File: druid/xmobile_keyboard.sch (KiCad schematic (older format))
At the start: 34 parts

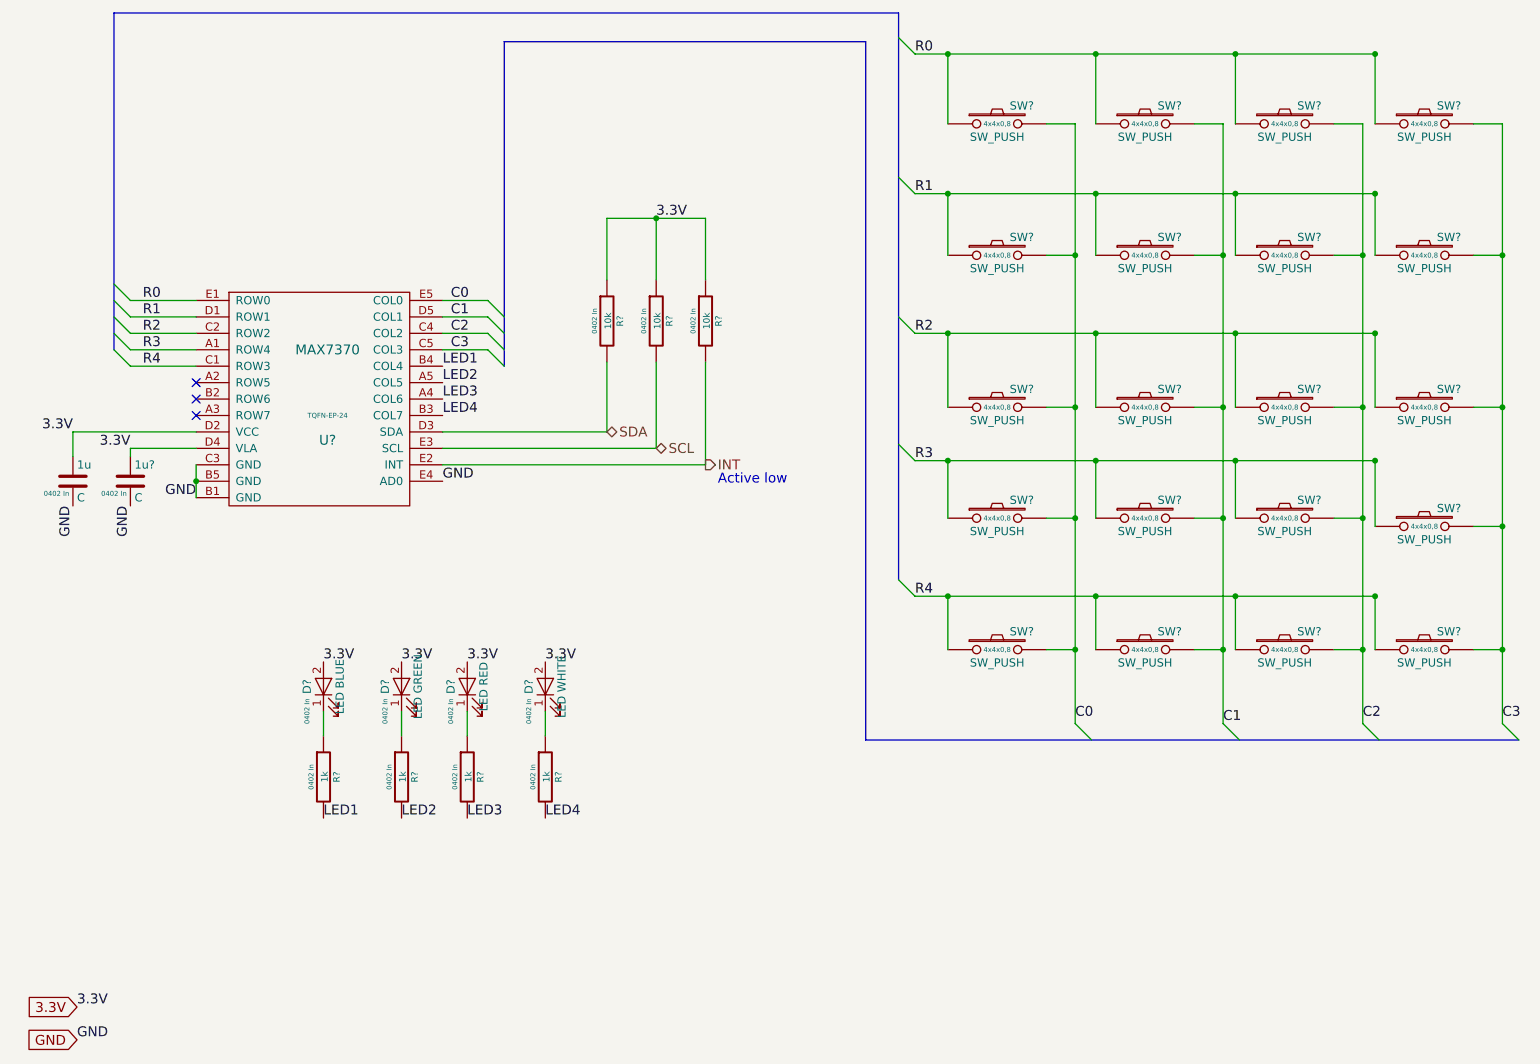
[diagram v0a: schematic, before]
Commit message: looks like all packages added.
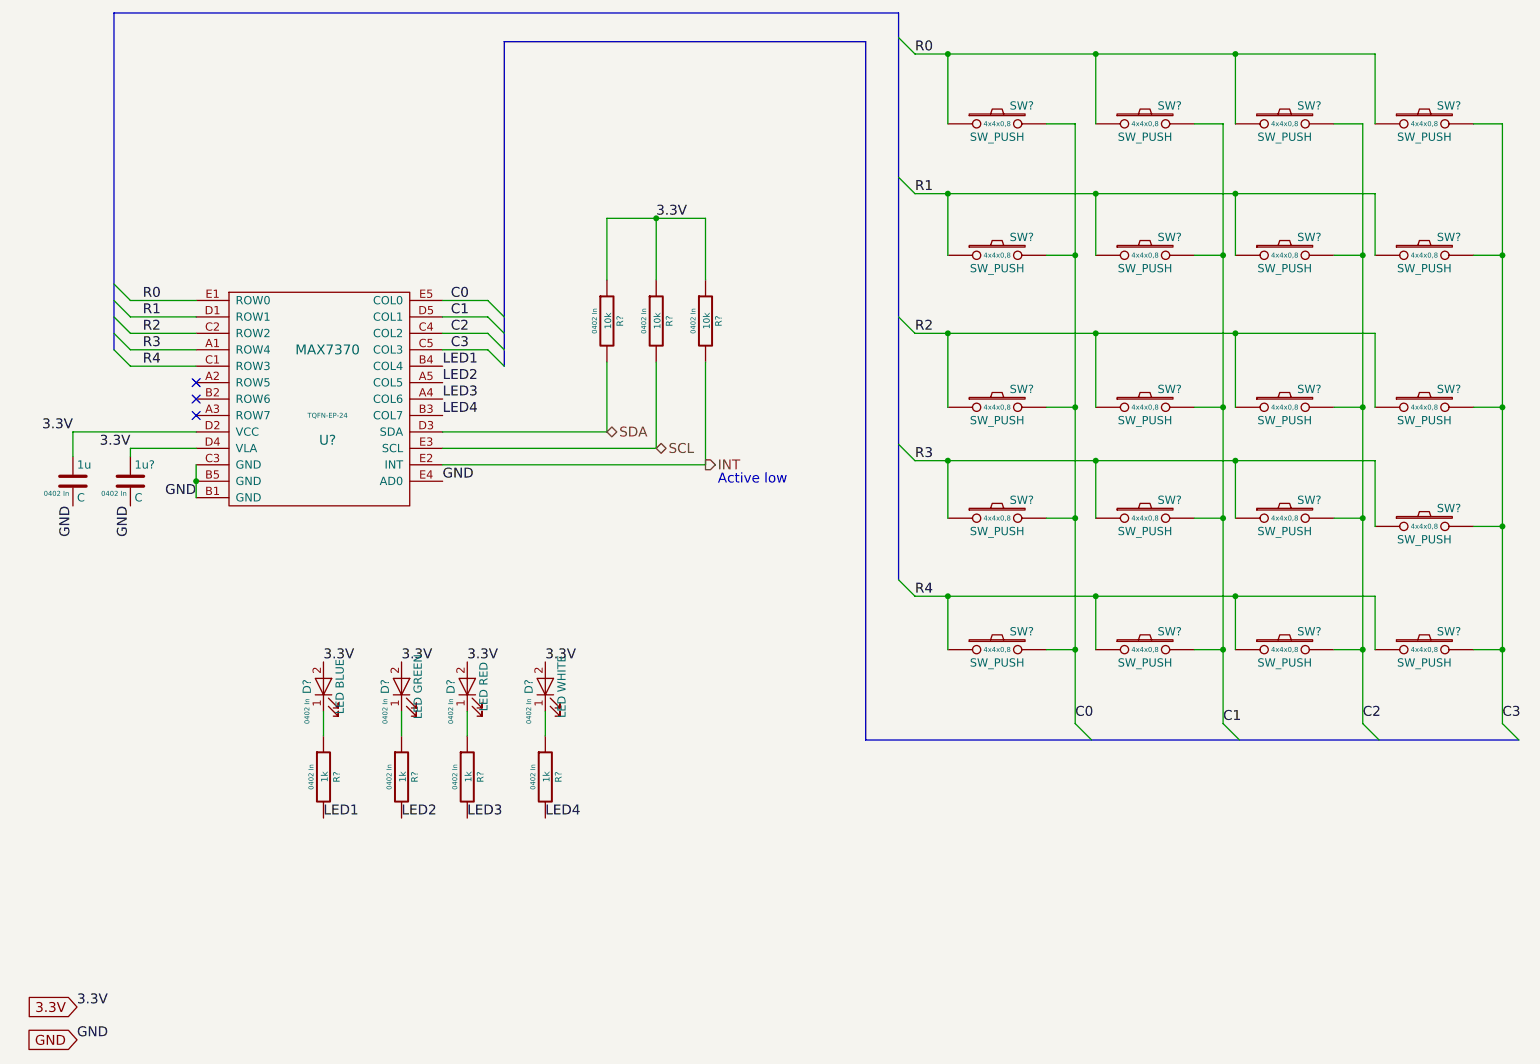
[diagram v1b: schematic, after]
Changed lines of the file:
@@
 Wire Wire Line
 	8975 1550 8975 1975
-Connection ~ 8975 1550
-Wire Wire Line
-	7150 1975 7150 5625
-Wire Wire Line
-	8050 1975 8050 5625
-Wire Wire Line
-	8900 1975 8900 5625
+Wire Wire Line
+	7150 1975 7150 2775
+Wire Wire Line
+	8050 1975 8050 2775
+Wire Wire Line
+	8900 1975 8900 2775
 Wire Wire Line
 	6375 2775 6375 2400
@@
 Wire Wire Line
 	8975 2400 8975 2775
-Connection ~ 8975 2400
 Wire Wire Line
 	8975 3250 8975 3700
-Connection ~ 8975 3250
 Wire Wire Line
 	6375 4375 6375 4025
@@
 Wire Wire Line
 	8975 4025 8975 4425
-Connection ~ 8975 4025
 Wire Wire Line
 	6375 5175 6375 4850
@@
 Wire Wire Line
 	8975 4850 8975 5175
-Connection ~ 8975 4850
-Wire Wire Line
-	6175 1550 8975 1550
-Wire Wire Line
-	6175 2400 8975 2400
-Wire Wire Line
-	6175 3250 8975 3250
-Wire Wire Line
-	6175 4025 8975 4025
-Wire Wire Line
-	6175 4850 8975 4850
-Wire Bus Line
-	6075 1300 6075 4750
+Wire Wire Line
+	6175 1550 6375 1550
+Wire Wire Line
+	6175 2400 6375 2400
+Wire Wire Line
+	6175 3250 6375 3250
+Wire Wire Line
+	6175 4025 6375 4025
+Wire Wire Line
+	6175 4850 6375 4850
 Wire Bus Line
 	1300 1300 6075 1300
@@
 Wire Wire Line
 	3300 3350 3575 3350
-Wire Bus Line
-	9850 5725 5875 5725
 Wire Bus Line
 	5875 5725 5875 1475
 Wire Bus Line
 	5875 1475 3675 1475
-Wire Bus Line
-	3675 1475 3675 3450
-Wire Bus Line
-	1300 1300 1300 3350
-Wire Wire Line
-	1800 4050 1800 4250
+Wire Wire Line
+	1800 4050 1800 4150
 Connection ~ 1800 4150
 Wire Wire Line
-	4300 2550 4900 2550
+	4300 2550 4600 2550
 Wire Wire Line
 	4300 2550 4300 2925
@@
 Connection ~ 9750 5175
 Wire Wire Line
-	9750 1975 9750 5625
+	9750 1975 9750 2775
 $Comp
 L xmobile-rescue:SW_PUSH SW?
@@
 	1    0    0    -1
 $EndComp
+Wire Wire Line
+	6375 1550 7275 1550
+Wire Wire Line
+	7275 1550 8125 1550
+Wire Wire Line
+	8125 1550 8975 1550
+Wire Wire Line
+	6375 2400 7275 2400
+Wire Wire Line
+	7275 2400 8125 2400
+Wire Wire Line
+	6375 3250 7275 3250
+Wire Wire Line
+	7275 3250 8125 3250
+Wire Wire Line
+	8125 3250 8975 3250
+Wire Wire Line
+	8125 2400 8975 2400
+Wire Wire Line
+	6375 4025 7275 4025
+Wire Wire Line
+	7275 4025 8125 4025
+Wire Wire Line
+	8125 4025 8975 4025
+Wire Wire Line
+	6375 4850 7275 4850
+Wire Wire Line
+	7275 4850 8125 4850
+Wire Wire Line
+	8125 4850 8975 4850
+Wire Wire Line
+	1800 4150 1800 4250
+Wire Wire Line
+	4600 2550 4900 2550
+Wire Wire Line
+	7150 3700 7150 4375
+Wire Wire Line
+	8050 3700 8050 4375
+Wire Wire Line
+	8900 3700 8900 4375
+Wire Wire Line
+	9750 3700 9750 4425
+Wire Wire Line
+	9750 2775 9750 3700
+Wire Wire Line
+	8900 2775 8900 3700
+Wire Wire Line
+	8050 2775 8050 3700
+Wire Wire Line
+	7150 2775 7150 3700
+Wire Wire Line
+	9750 4425 9750 5175
+Wire Wire Line
+	8900 4375 8900 5175
+Wire Wire Line
+	8050 4375 8050 5175
+Wire Wire Line
+	7150 4375 7150 5175
+Wire Wire Line
+	7150 5175 7150 5625
+Wire Wire Line
+	8050 5175 8050 5625
+Wire Wire Line
+	8900 5175 8900 5625
+Wire Wire Line
+	9750 5175 9750 5625
+Wire Bus Line
+	5875 5725 9850 5725
+Wire Bus Line
+	3675 1475 3675 3450
+Wire Bus Line
+	1300 1300 1300 3350
+Wire Bus Line
+	6075 1300 6075 4750
 $EndSCHEMATC
